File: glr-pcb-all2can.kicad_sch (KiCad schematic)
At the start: 45 parts, among them IC2 ZMR330FTA, IC3 AP64060WU-7, IC4 STM32C092KCT6, IC5 AP64060WU-7, J1 Conn_02x02_Counter_Clockwise_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, J2 Conn_02x02_Counter_Clockwise_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, J3 Conn_02x02_Counter_Clockwise_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, J4 Conn_02x02_Counter_Clockwise_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, J5 Conn_01x04, J6 Conn_01x02, J7 Conn_01x02, J8 62701021621

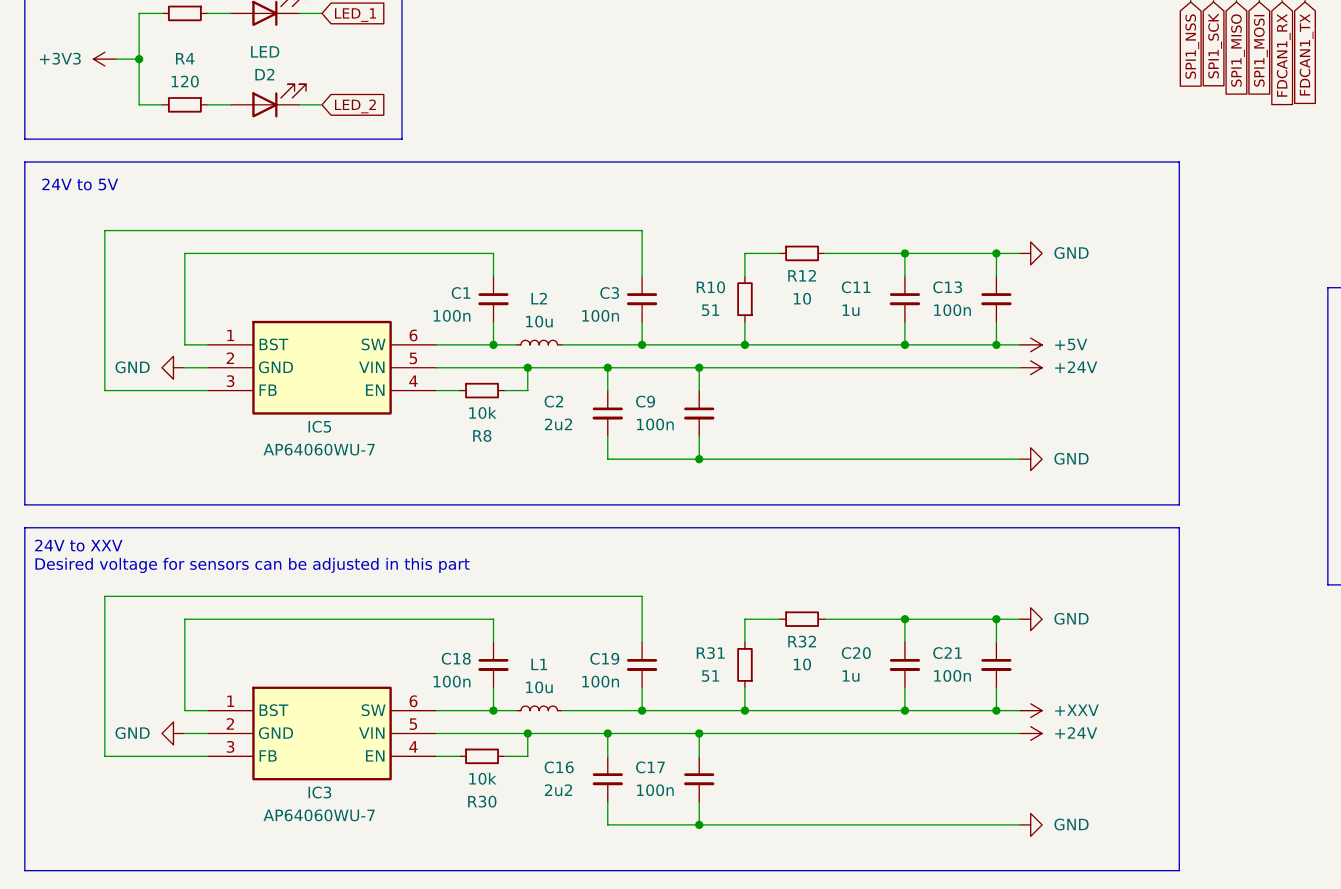
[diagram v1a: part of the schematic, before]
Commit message: update buck converters
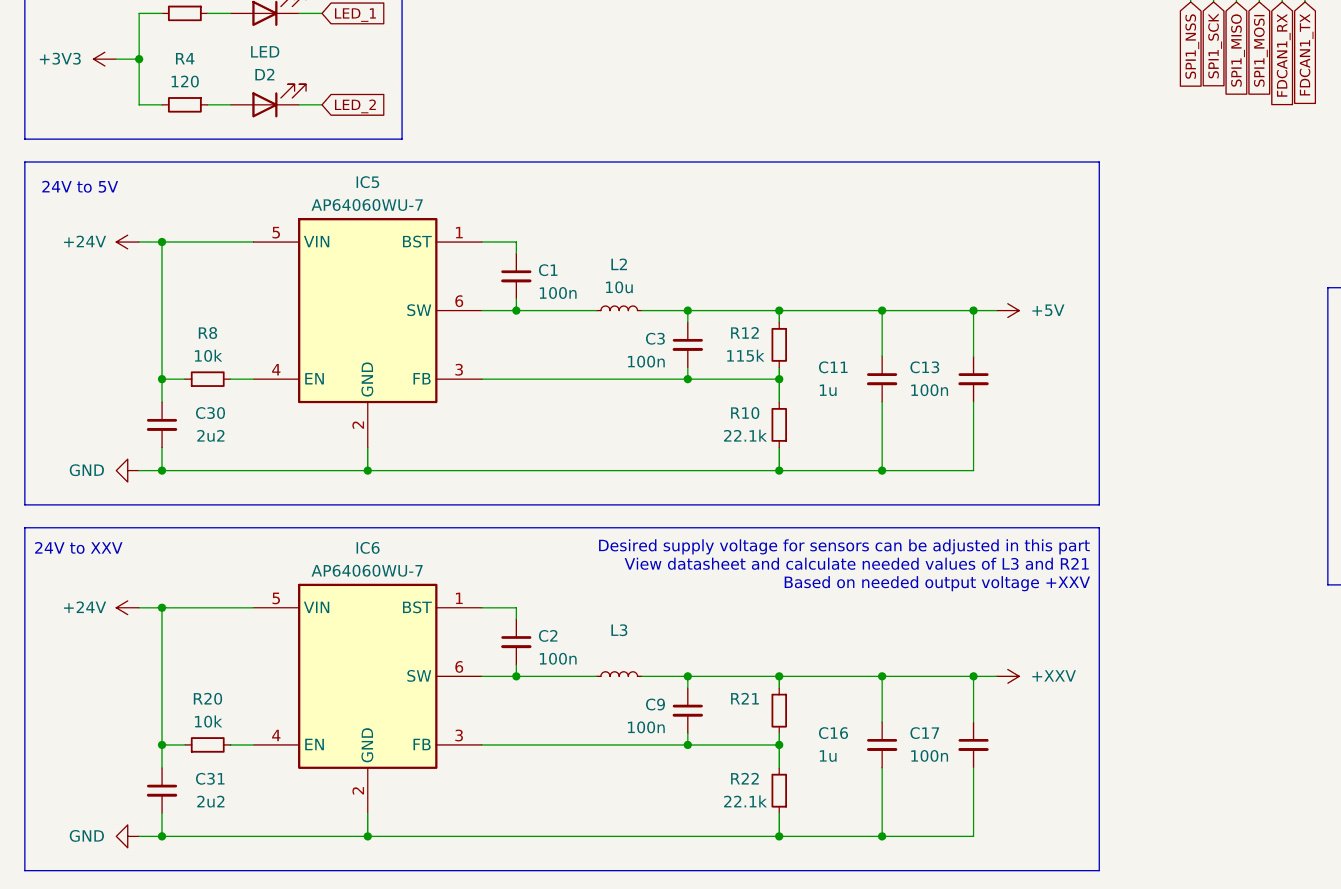
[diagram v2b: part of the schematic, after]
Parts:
- removed C18, C19, C21: 100n, Capacitor_SMD:C_0603_1608Metric, symbol Device:C_Small
- removed C20: 1u, Capacitor_SMD:C_0603_1608Metric, symbol Device:C_Small
- removed IC3: AP64060WU-7, SamacSys_Parts:SOT95P280X100-6N, symbol SamacSys_Parts:AP64060WU-7
- removed L1: 10u, Inductor_SMD:L_1008_2520Metric, symbol Device:L_Small
- removed R30: 10k, Resistor_SMD:R_0603_1608Metric, symbol Device:R_Small
- removed R31: 51, Resistor_SMD:R_0603_1608Metric, symbol Device:R_Small
- removed R32: 10, Resistor_SMD:R_0603_1608Metric, symbol Device:R_Small
- added C30, C31: 2u2, Capacitor_SMD:C_0603_1608Metric, symbol Device:C_Small
- added IC6: AP64060WU-7, SOT95P280X100-6N, symbol SamacSys_Parts:AP64060WU-7
- added L3: ~, Inductor_SMD:L_1008_2520Metric, symbol Device:L_Small
- added R20: 10k, Resistor_SMD:R_0603_1608Metric, symbol Device:R_Small
- added R21: ~, Resistor_SMD:R_0603_1608Metric, symbol Device:R_Small
- added R22: 22.1k, Resistor_SMD:R_0603_1608Metric, symbol Device:R_Small
- C16: value 2u2 -> 1u
- C2: value 2u2 -> 100n
- IC5: footprint SamacSys_Parts:SOT95P280X100-6N -> SOT95P280X100-6N
- R10: value 51 -> 22.1k
- R12: value 10 -> 115k
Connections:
- net +24V: now also R8.1, C30.1, C31.1, IC6.5 (VIN), R20.1; no longer C16.1, C17.1, C2.1, C9.1, R8.2
- net +5V: now also C11.1, C13.1, C3.1, R12.1; no longer C11.2, C13.2, C3.2, R10.1
- net +XXV: now also C16.1, C17.1, C9.1, L3.2, R21.1
- net GND: now also C11.2, C13.2, R10.1, C30.2, C31.2, IC6.2 (GND), R22.1; no longer C11.1, C13.1, C2.2, C9.2, R12.2
- net at IC5.3 (FB): now also C3.2, R10.2, R12.2; no longer C3.1
- net at IC5.4 (EN): now also R8.2; no longer R8.1
- new net: C2.1, IC6.1 (BST)
- new net: C2.2, IC6.6 (SW), L3.1
- new net: C9.2, IC6.3 (FB), R21.2, R22.2
- new net: IC6.4 (EN), R20.2
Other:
- note added: "24V to XXV"
- note added: "Desired supply voltage for sensors can be adjusted in this part View datasheet and calculate needed values of L3 and R21 Based on needed output voltage +XXV"
- note removed: "24V to XXV Desired voltage for sensors can be adjusted in this part"
